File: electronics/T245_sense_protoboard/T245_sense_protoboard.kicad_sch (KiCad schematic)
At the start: 2 parts

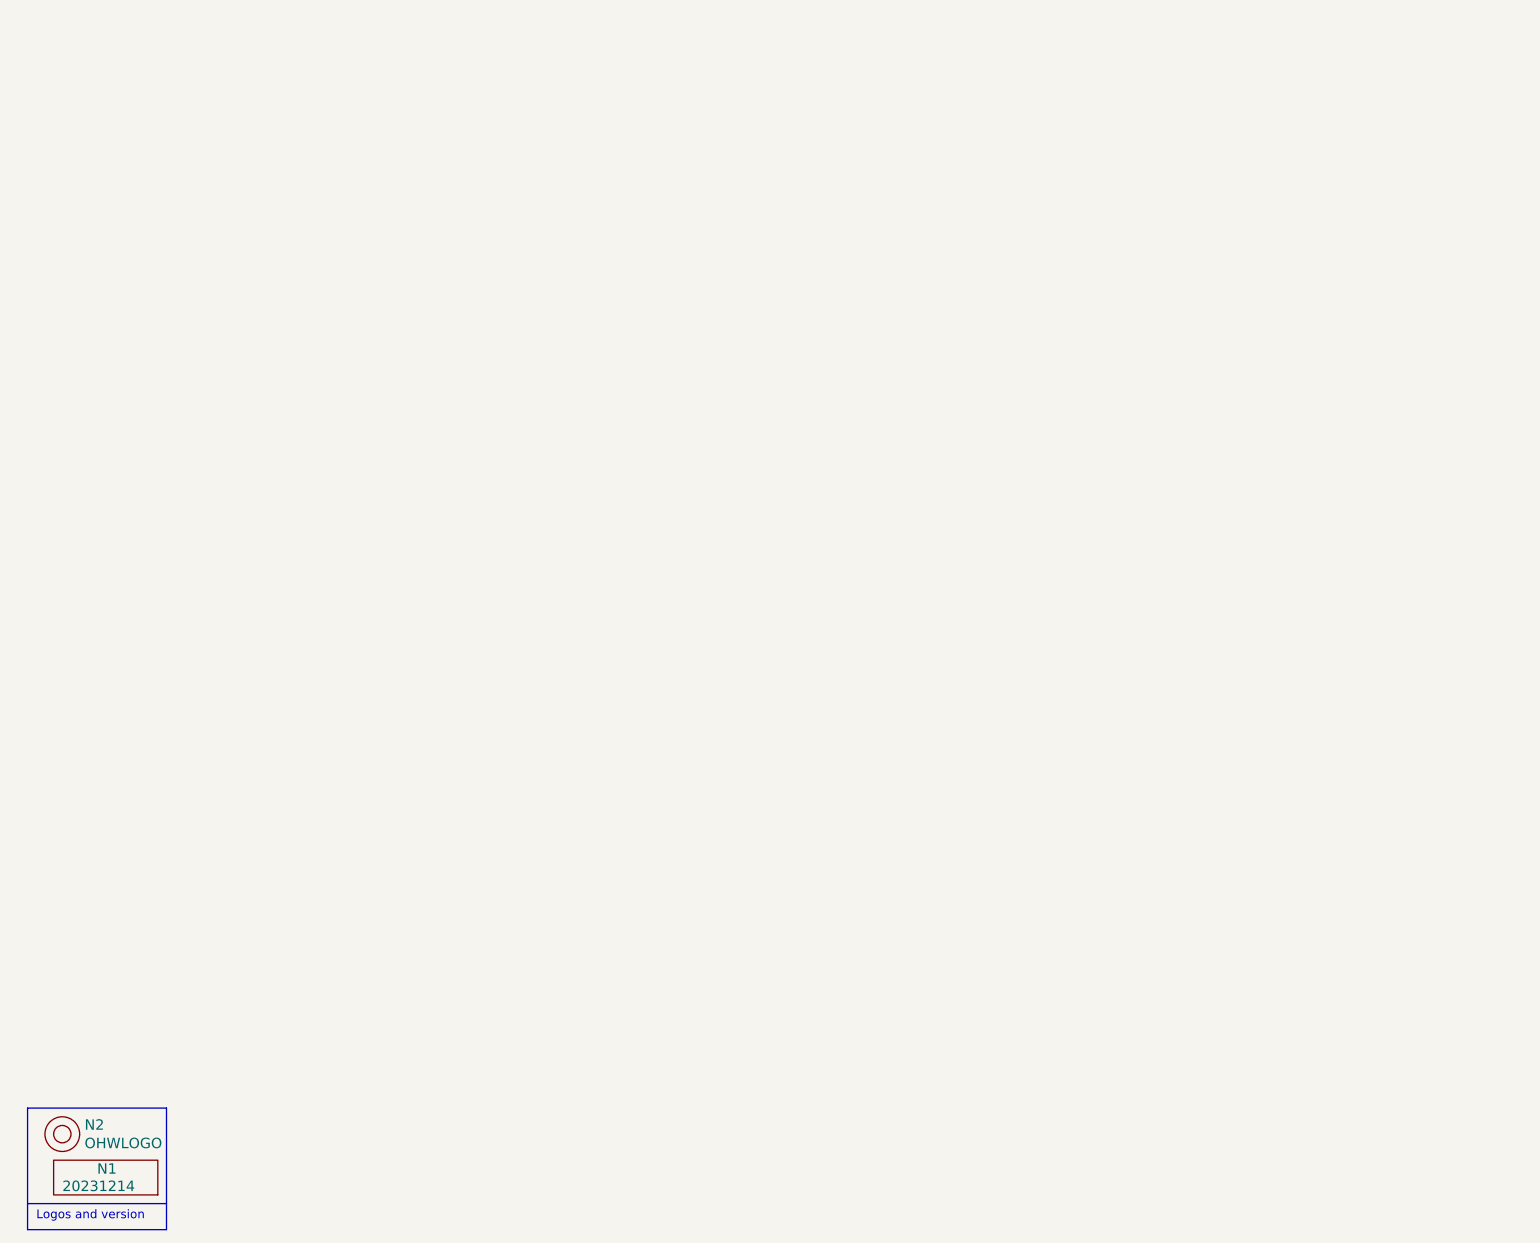
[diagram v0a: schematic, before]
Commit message: WIP placement
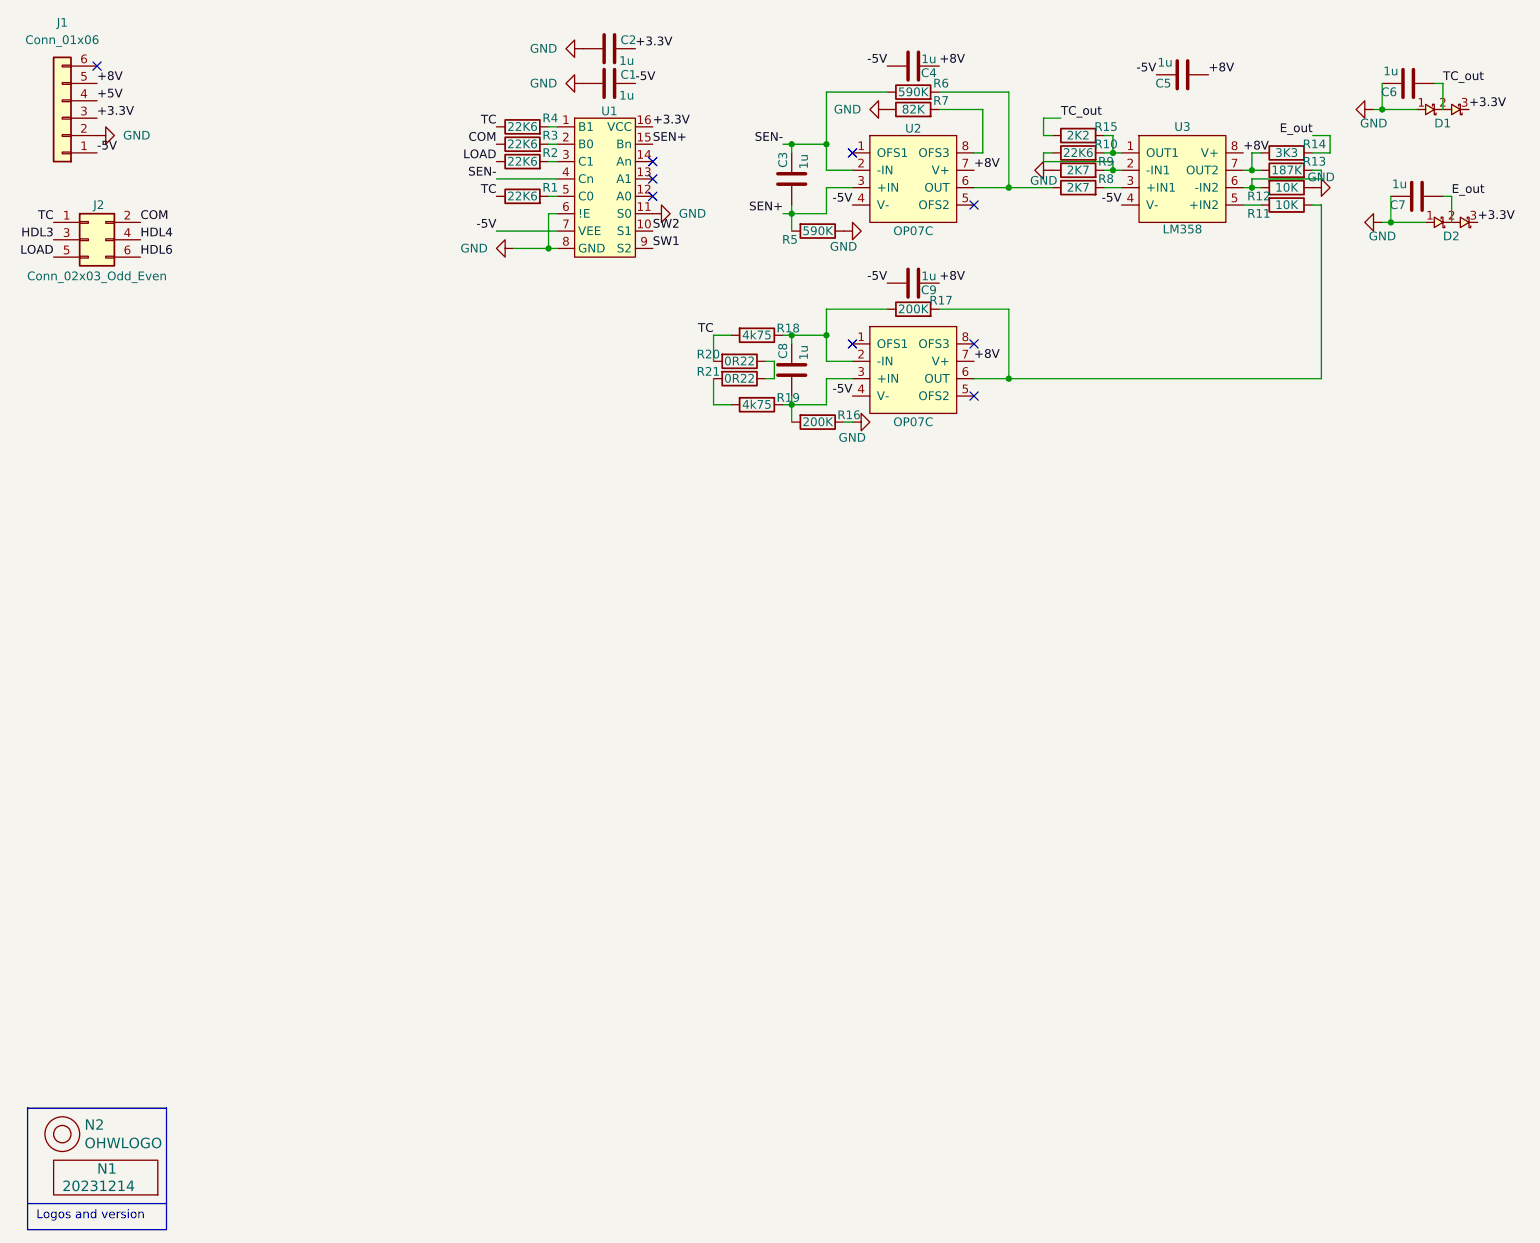
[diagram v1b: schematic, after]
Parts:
- added C1, C2, C3, C4, C5, C6, C7, C8, C9: 1u, SquantorCapacitor:C_0603, symbol Device:C
- added D1, D2: ~, SquantorIC:SOT23-3, symbol SquantorDiodes:shottky_series
- added J1: Conn_01x06, Connector_Molex:Molex_KK-254_AE-6410-06A_1x06_P2.54mm_Vertical, symbol Connector_Generic:Conn_01x06
- added J2: Conn_02x03_Odd_Even, Connector_Molex:Molex_Micro-Fit_3.0_43045-0612_2x03_P3.00mm_Vertical, symbol Connector_Generic:Conn_02x03_Odd_Even
- added R1, R10, R2, R3, R4: 22K6, SquantorResistor:R_0603_hand, symbol Device:R
- added R11, R12: 10K, SquantorResistor:R_0603_hand, symbol Device:R
- added R13: 187K, SquantorResistor:R_0603_hand, symbol Device:R
- added R14: 3K3, SquantorResistor:R_0603_hand, symbol Device:R
- added R15: 2K2, SquantorResistor:R_0603_hand, symbol Device:R
- added R16, R17: 200K, SquantorResistor:R_0603_hand, symbol Device:R
- added R18, R19: 4k75, SquantorResistor:R_0603_hand, symbol Device:R
- added R20, R21: 0R22, SquantorResistor:R_0805, symbol Device:R
- added R5, R6: 590K, SquantorResistor:R_0603_hand, symbol Device:R
- added R7: 82K, SquantorResistor:R_0603_hand, symbol Device:R
- added R8, R9: 2K7, SquantorResistor:R_0603_hand, symbol Device:R
- added U1: ~, Package_DIP:DIP-16_W7.62mm, symbol SquantorLogic:74XX4053
- added U2, U4: OP07C, Package_DIP:DIP-8_W7.62mm, symbol SquantorGenericAnalog:opamp_single_8pin
- added U3: LM358, Package_DIP:DIP-8_W7.62mm, symbol SquantorGenericAnalog:opamp_dual_8pin
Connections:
- new net: R6.2, R8.1, U2.6 (OUT)
- new net: R7.2, U2.8 (OFS3)
- new net: R1.2, U1.5 (C0)
- new net: R10.1, R9.2, U3.2 (-IN1)
- new net: C8.1, R16.2, R19.1, U4.3 (+IN)
- new net: R19.2, R21.2
- new net: R3.2, U1.2 (B0)
- new net: R20.1, R21.1
- new net: R10.2, R15.2, U3.1 (OUT1)
- new net: R11.1, R17.2, U4.6 (OUT)
- new net: R11.2, U3.5 (+IN2)
- new net: C8.2, R17.1, R18.1, U4.2 (-IN)
- new net: R13.1, R14.1, U3.7 (OUT2)
- new net: R4.2, U1.1 (B1)
- new net: R12.2, R13.2, U3.6 (-IN2)
- new net: R8.2, U3.3 (+IN1)
- new net: R2.2, U1.3 (C1)
- new net +3.3V: C2.2, D1.3, D2.3, J1.3 (Pin_3), U1.16 (VCC)
- new net +5V: J1.4 (Pin_4)
- new net +8V: C4.1, C5.1, C9.1, J1.5 (Pin_5), U2.7 (V+), U3.8 (V+), U4.7 (V+)
- new net -5V: C1.2, C4.2, C5.2, C9.2, J1.1 (Pin_1), U1.7 (VEE), U2.4 (V-), U3.4 (V-), U4.4 (V-)
- new net COM: J2.2 (Pin_2), R3.1
- new net E_out: C7.1, D2.2, R14.2
- new net GND: C1.1, C2.1, C6.2, C7.2, D1.1, D2.1, J1.2 (Pin_2), R12.1, R16.1, R5.1, R7.1, R9.1, U1.11 (S0), U1.6 (!E), U1.8 (GND)
- new net HDL3: J2.3 (Pin_3)
- new net HDL4: J2.4 (Pin_4)
- new net HDL6: J2.6 (Pin_6)
- new net LOAD: J2.5 (Pin_5), R2.1
- new net SEN+: C3.1, R5.2, U1.15 (Bn), U2.3 (+IN)
- new net SEN-: C3.2, R6.1, U1.4 (Cn), U2.2 (-IN)
- new net SW1: U1.9 (S2)
- new net SW2: U1.10 (S1)
- new net TC: J2.1 (Pin_1), R1.1, R18.2, R20.2, R4.1
- new net TC_out: C6.1, D1.2, R15.1
- no-connect marks 0 -> 9
